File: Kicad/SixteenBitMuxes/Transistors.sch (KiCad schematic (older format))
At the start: 20 parts, among them Q1 PN2222A, Q10 2SC1815, Q12 S9013, Q14 S9018, Q15 BC848B, Q16 2SC1623, Q17 MPSA18, Q19 2N5088, Q2 MMBT3904, Q3 MMBT5551L, Q4 MMBTA42, Q5 BC807, Q6 BC846, Q7 BC847B, Q8 BC847C, Q9 C945, U8 CD4067BM, U9 CD4067BM

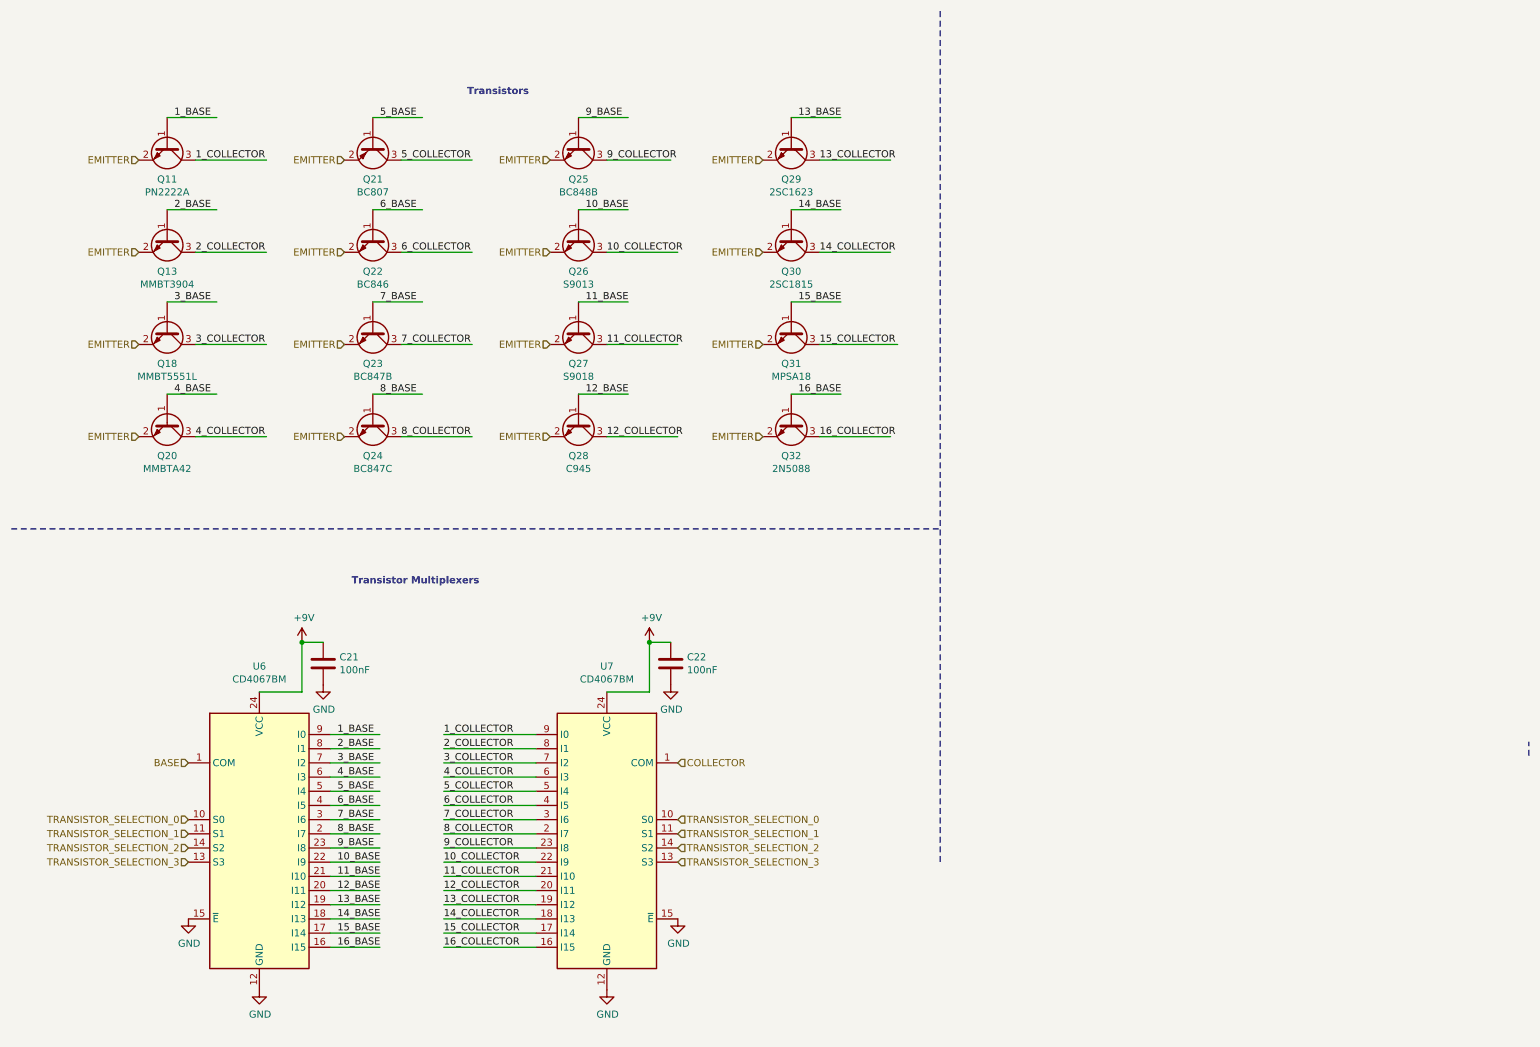
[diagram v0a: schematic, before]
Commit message: EEprom + PCB changes
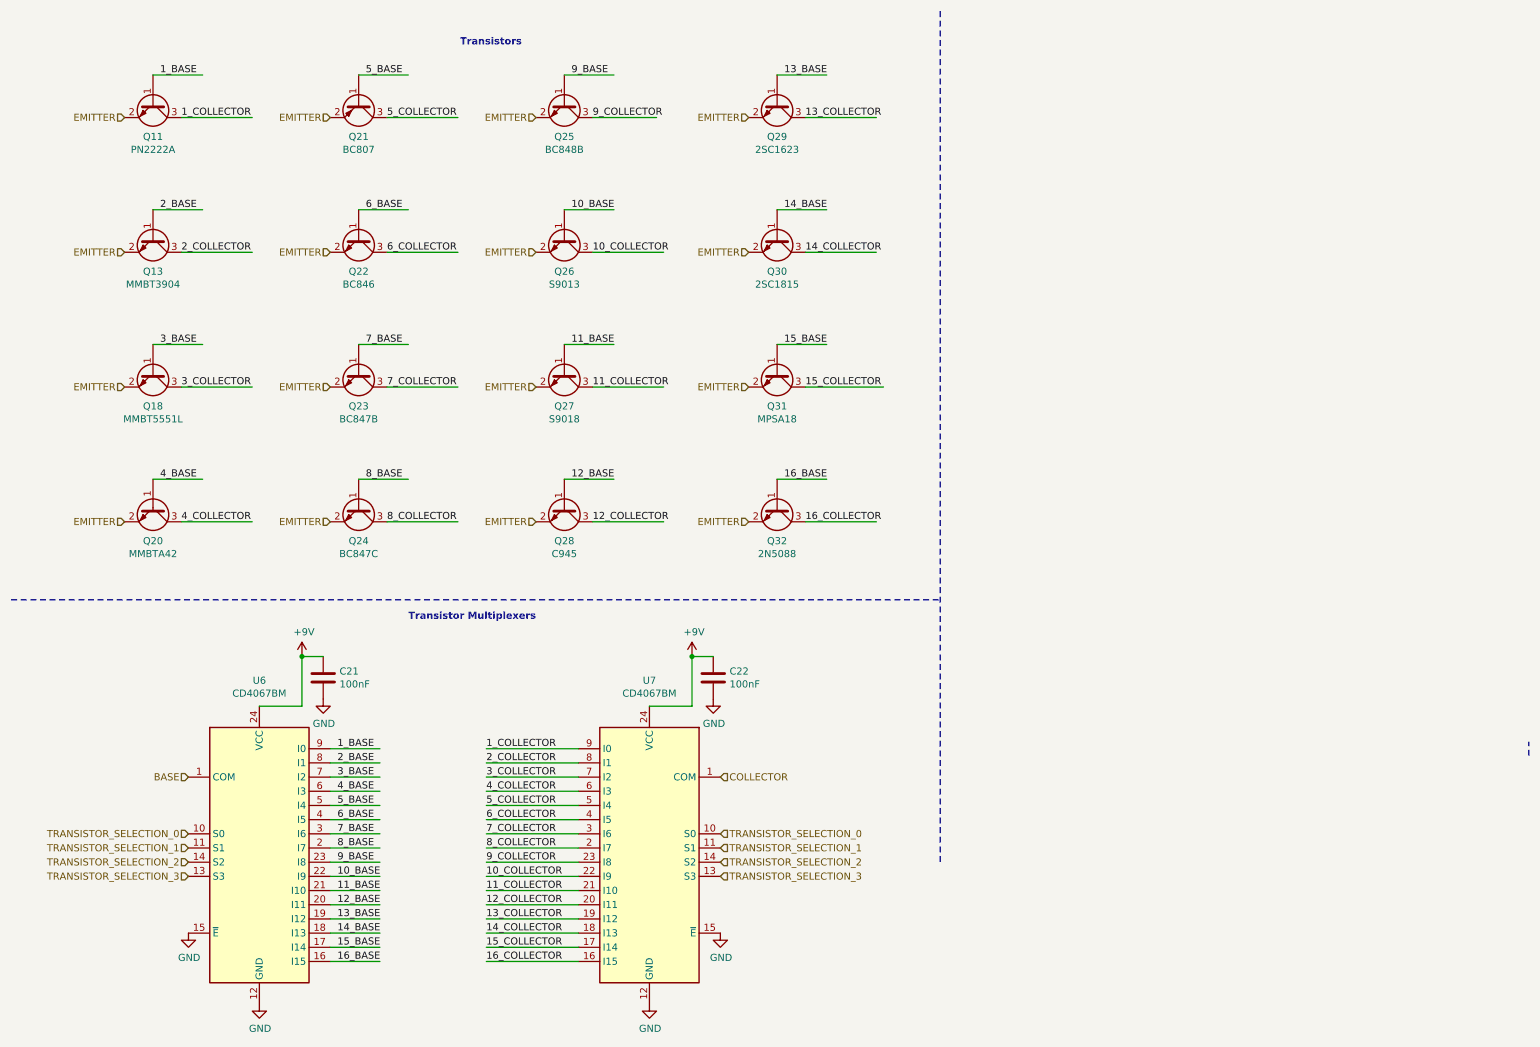
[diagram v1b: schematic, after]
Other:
- moved on the sheet: C21, C22, Q11, Q13, Q18, Q20, Q21, Q22, Q23, Q24, Q25, Q26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
